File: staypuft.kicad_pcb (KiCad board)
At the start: 2 copper layers, 68 x 77.5 mm, 53 parts, among them J1 Conn_01x04_Male, Q1 2N5088, Q2 2N5088, Q3 2N5088, Q4 2N5088

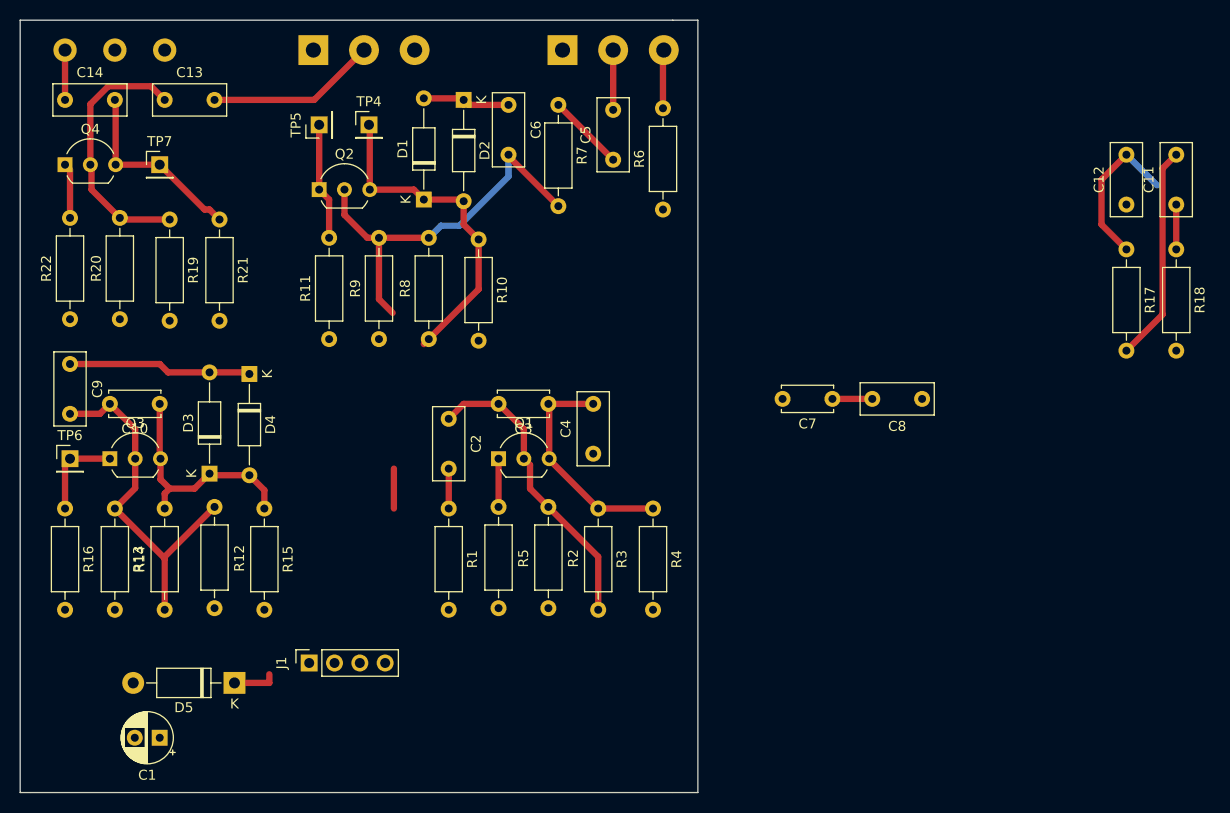
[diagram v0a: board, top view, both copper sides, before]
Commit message: rough pcb done, align todo
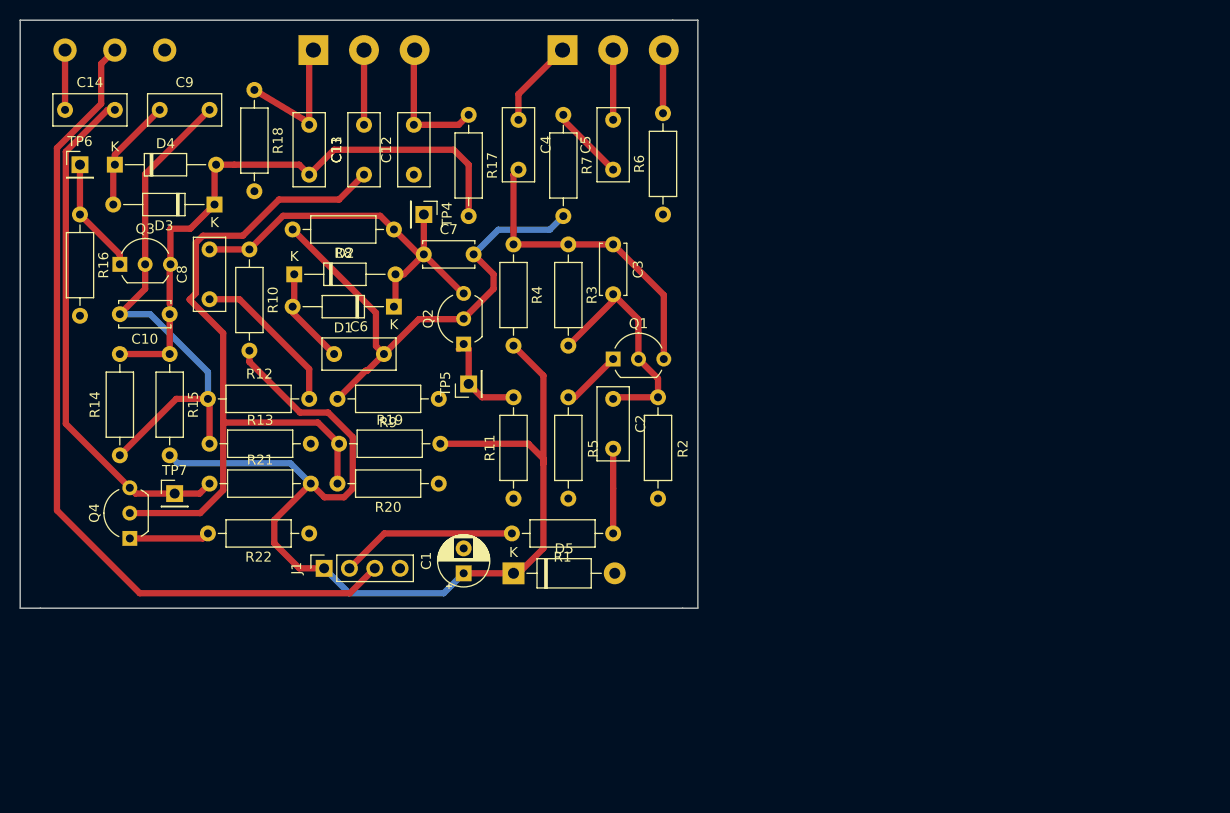
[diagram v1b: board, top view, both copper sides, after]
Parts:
- moved R18 93.9 mm to (141.0, 73.0)
- moved C11 87.4 mm to (146.5, 76.5), turned to 270 degrees
- moved C8 72.2 mm to (136.5, 94.0), turned to 90 degrees
- moved C12 71.6 mm to (157.0, 81.5)
- moved R17 67.4 mm to (162.5, 75.5)
- moved C7 43.5 mm to (158.0, 89.5), turned to 0 degrees
- moved Q4 38.1 mm to (128.5, 118.0), turned to 90 degrees
- moved R20 36.0 mm to (159.5, 112.5), turned to 180 degrees
- moved C1 34.7 mm to (162.0, 121.5), turned to 90 degrees
- moved C4 34.3 mm to (167.5, 76.0), turned to 270 degrees
- moved TP7 33.0 mm to (133.0, 113.5)
- moved R22 32.2 mm to (146.5, 117.5), turned to 180 degrees
- moved C6 30.5 mm to (149.0, 99.5), turned to 0 degrees
- moved D5 30.1 mm to (167.0, 121.5), turned to 0 degrees
- moved TP5 30.0 mm to (162.5, 102.5)
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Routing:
- net pwr: track 4.37 -> 111.8 mm
- net out: track 0.00 -> 85.0 mm
- net Net-(C13-Pad1): track 26.5 -> 73.1 mm
- net Net-(C14-Pad2): track 19.2 -> 51.9 mm
- net Net-(C10-Pad2): track 36.3 -> 53.9 mm
- net in: track 0.27 -> 17.7 mm
- net Net-(C8-Pad1): track 0.00 -> 15.9 mm
- net Net-(C10-Pad1): track 45.5 -> 58.7 mm
- net Net-(C6-Pad2): track 40.0 -> 51.4 mm
- net Net-(C11-Pad1): track 4.50 -> 14.2 mm
- net Net-(C13-Pad2): track 17.1 -> 7.50 mm
- net Net-(C4-Pad1): track 0.00 -> 8.83 mm
- net Net-(C3-Pad1): track 22.6 -> 31.3 mm
- net Net-(C9-Pad1): track 18.4 -> 11.4 mm
- net Net-(C2-Pad1): track 30.4 -> 23.8 mm
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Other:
- board size 68 x 77.5 mm -> 68 x 59 mm
